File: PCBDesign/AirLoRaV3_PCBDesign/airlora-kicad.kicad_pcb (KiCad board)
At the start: 4 copper layers, 60 x 60 mm, 87 parts, among them IC1 BALFHB-WL-05D3, J1 12V, J2 Conn_Coaxial, J3 DHT, J4 UART1, J5 UART2, J6 I2C, J7 UART2, Q1 S8050, Q2 S8050, Q3 S8050, Q4 S8050, SW1 SW_Push, U1 TPS54202DDC, U2 TPS7A2633DRVR, U3 BGS12WN6E6327, U4 STM32WLE5JCIx, Y1 NX2012SA 32.768KHz

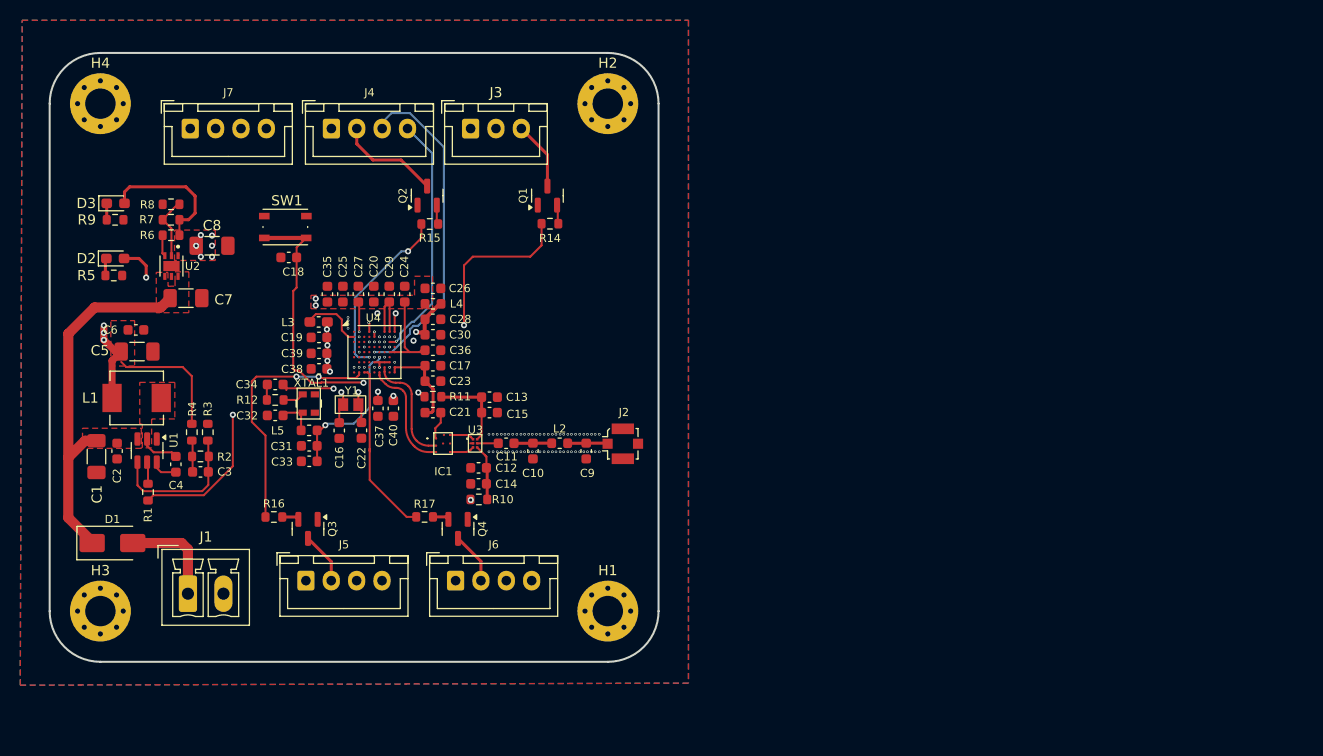
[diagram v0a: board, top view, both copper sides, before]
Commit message: update
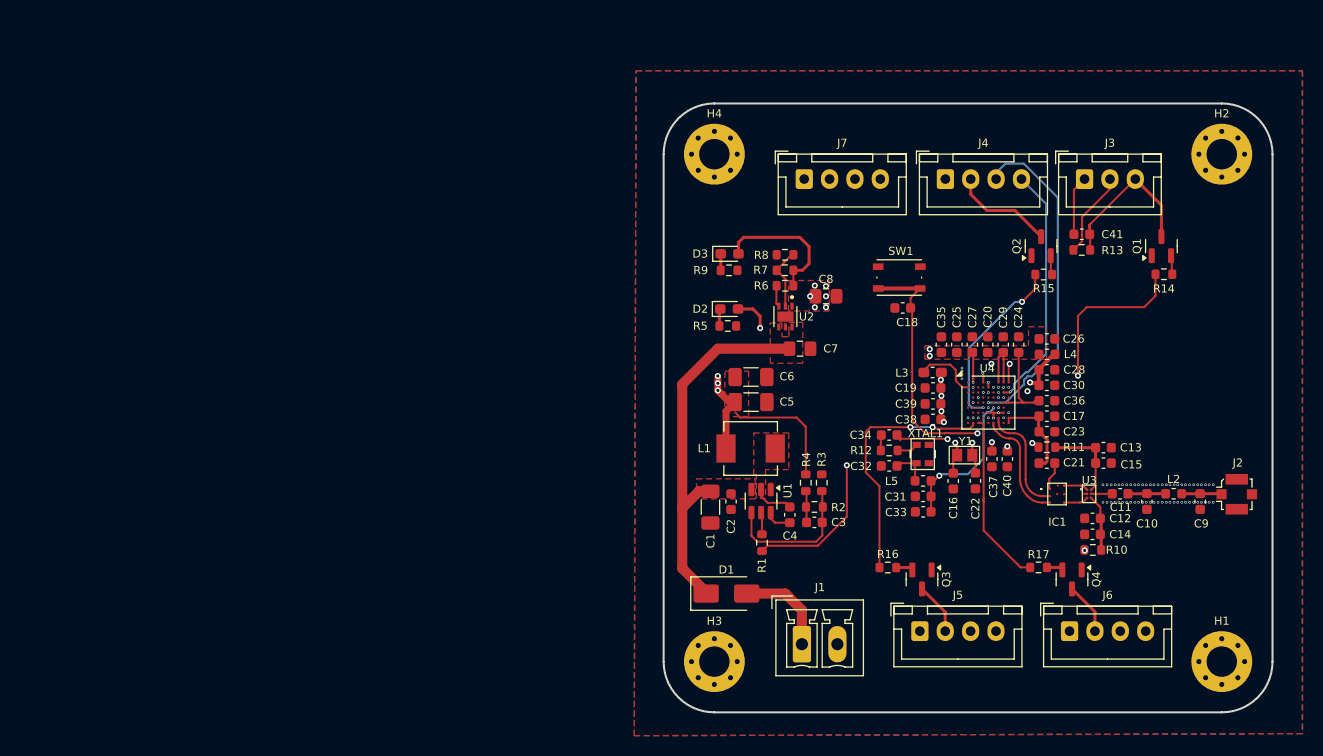
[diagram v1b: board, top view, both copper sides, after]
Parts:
- added C41: 0.1uF, Capacitor_SMD:C_0603_1608Metric, F.Cu at (165.7, 70.9)
- added R13: 1K, Resistor_SMD:R_0603_1608Metric, F.Cu at (165.7, 72.4)
- C6: footprint Capacitor_SMD:C_0603_1608Metric -> Capacitor_SMD:C_1206_3216Metric_Pad1.33x1.80mm_HandSolder
- C7, C8: footprint Capacitor_SMD:C_1206_3216Metric_Pad1.33x1.80mm_HandSolder -> Capacitor_SMD:C_0805_2012Metric_Pad1.18x1.45mm_HandSolder
- moved C6 60.8 mm to (133.1, 84.9)
- moved C1 60.7 mm to (129.1, 97.8)
- moved C5 60.7 mm to (133.1, 87.4)
- moved D2 60.7 mm to (131.0, 78.2)
- moved D3 60.7 mm to (131.0, 72.8)
- moved J2 60.7 mm to (181.0, 96.5)
- moved L1 60.7 mm to (133.1, 92.0)
- moved Q2 60.7 mm to (161.7, 72.0)
- moved Q3 60.7 mm to (150.0, 104.9)
- moved R6 60.7 mm to (136.5, 75.9)
- moved R7 60.7 mm to (136.5, 74.4)
- moved R8 60.7 mm to (136.5, 72.9)
- moved U3 60.7 mm to (166.4, 96.4)
- moved C10 60.7 mm to (172.1, 97.2)
- moved C11 60.7 mm to (169.5, 96.4)
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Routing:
- net Net-(J3-Pin_3): track 6.74 -> 16.8 mm
- net /AirLora V3/MCU/PA11: track 25.1 -> 33.6 mm
- net +5V: track 133.2 -> 139.1 mm
- net /AirLora V3/MCU/PA12: track 37.8 -> 42.7 mm
- net Net-(D1-A): track 10.1 -> 9.47 mm
- net 12V: track 36.5 -> 37.1 mm
- net Net-(U4-NRST): track 28.2 -> 27.7 mm
- net GND: vias 65 -> 66
- net /AirLora V3/MCU/PB14_SDA: vias 1 -> 0
